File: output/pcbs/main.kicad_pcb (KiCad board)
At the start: 2 copper layers, 142.8 x 177.6 mm, 63 parts

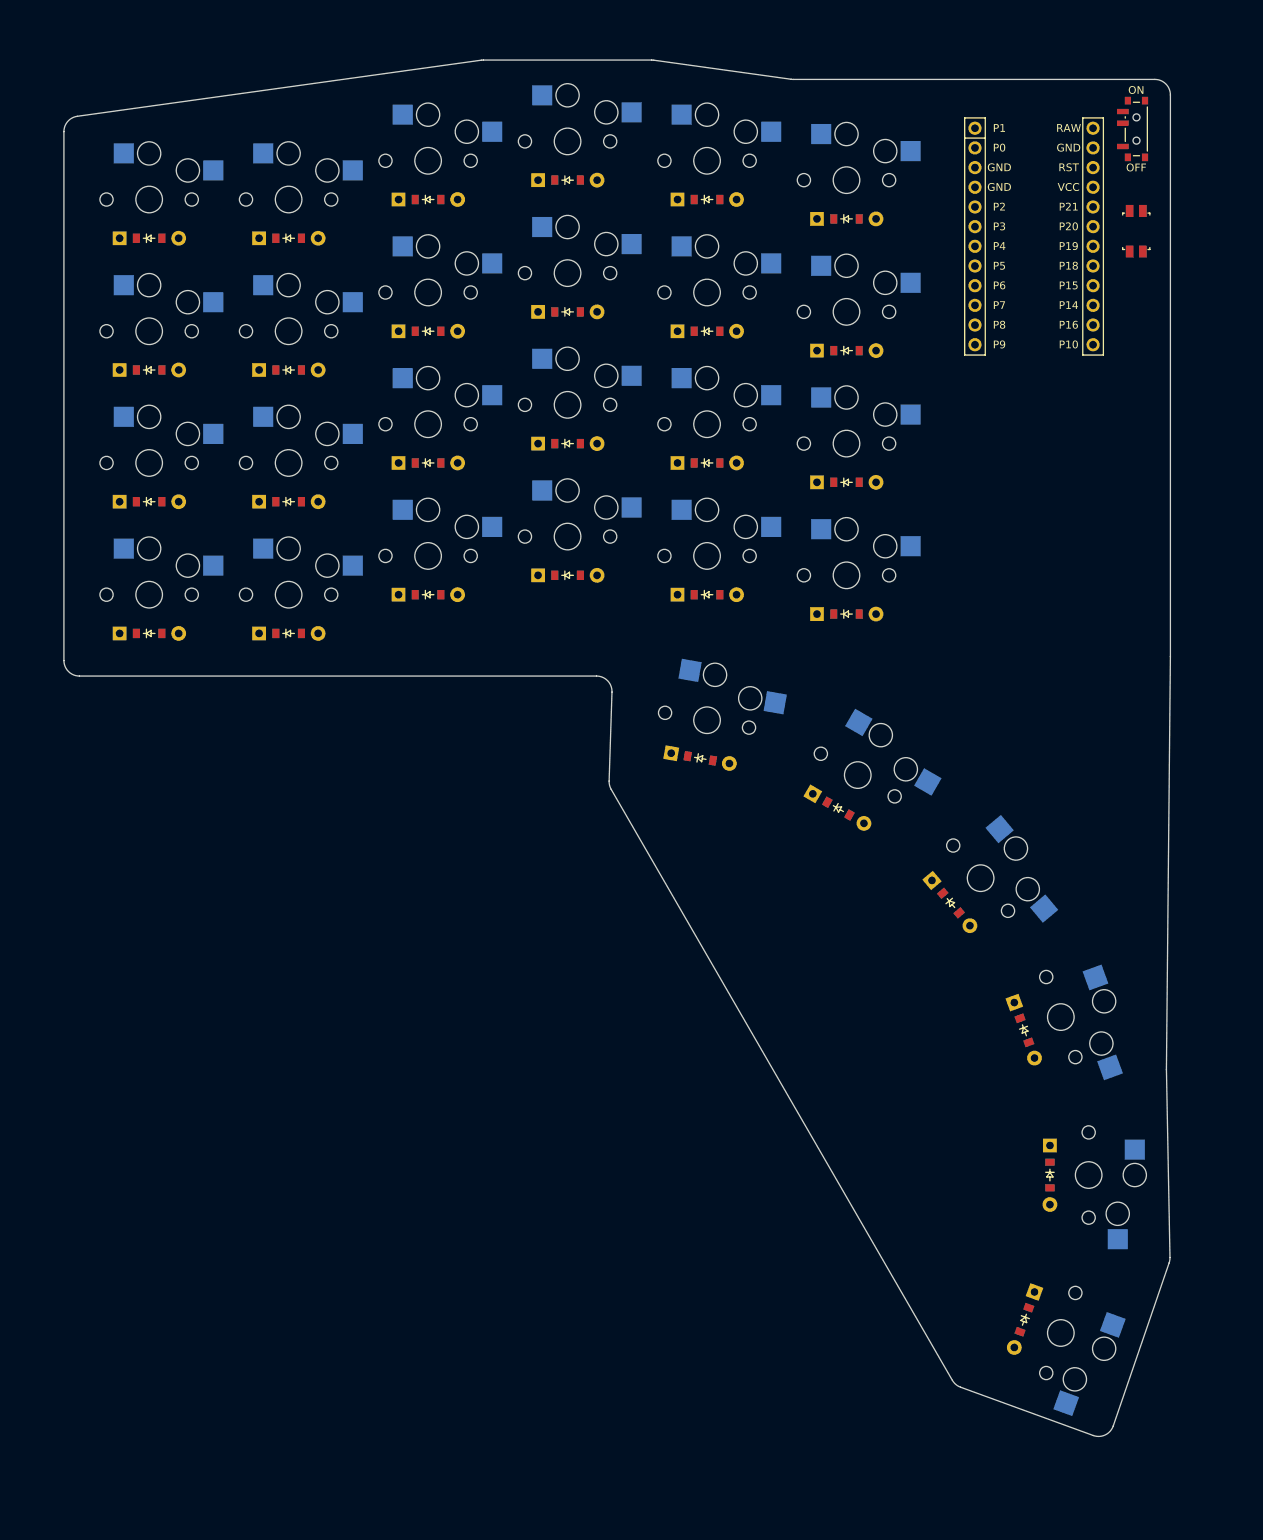
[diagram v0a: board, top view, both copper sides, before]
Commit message: Finished left half maybe
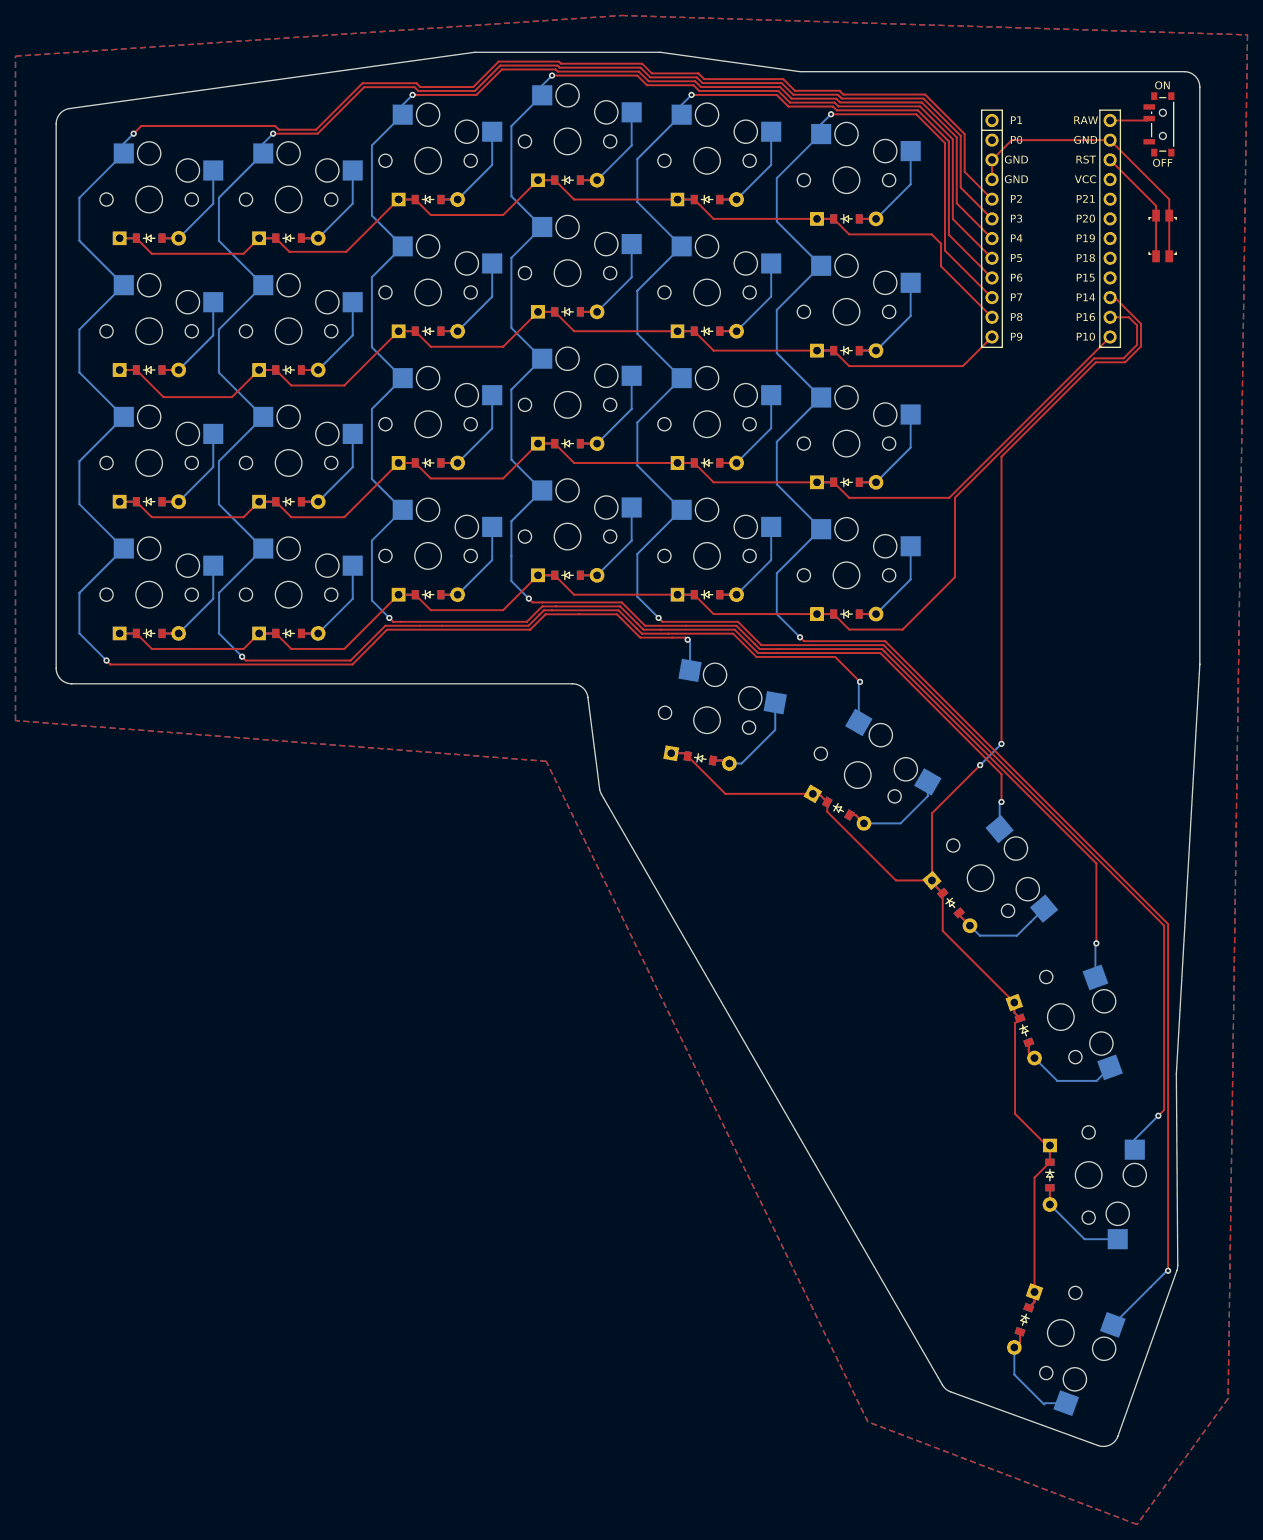
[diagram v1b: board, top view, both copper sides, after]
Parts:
- moved PWR1 3.45 mm to (230.8, 39.3)
- moved RST1 3.45 mm to (230.8, 53.7)
- moved MCU1 2.42 mm to (216.4, 51.5)
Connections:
- D1 pad 1: P5 -> P16
- D10 pad 1: P4 -> P10
- D11 pad 1: P3 -> P9
- D12 pad 1: P2 -> P8
- D13 pad 1: P5 -> P16
- D14 pad 1: P4 -> P10
- D15 pad 1: P3 -> P9
- D16 pad 1: P2 -> P8
- D17 pad 1: P5 -> P16
- D18 pad 1: P4 -> P10
- D19 pad 1: P3 -> P9
- D2 pad 1: P4 -> P10
- D20 pad 1: P2 -> P8
- D21 pad 1: P5 -> P16
- D22 pad 1: P4 -> P10
- D23 pad 1: P3 -> P9
- D24 pad 1: P2 -> P8
- D3 pad 1: P3 -> P9
- D4 pad 1: P2 -> P8
- D5 pad 1: P5 -> P16
- D6 pad 1: P4 -> P10
- D7 pad 1: P3 -> P9
- D8 pad 1: P2 -> P8
- D9 pad 1: P5 -> P16
- S1 pad 1: P6 -> P2
- S10 pad 1: P8 -> P4
- S11 pad 1: P8 -> P4
- S12 pad 1: P8 -> P4
- S13 pad 1: P9 -> P5
- S14 pad 1: P9 -> P5
- S15 pad 1: P9 -> P5
- S16 pad 1: P9 -> P5
- S17 pad 1: P10 -> P6
- S18 pad 1: P10 -> P6
- S19 pad 1: P10 -> P6
- S2 pad 1: P6 -> P2
- S20 pad 1: P10 -> P6
- S21 pad 1: P16 -> P7
- S22 pad 1: P16 -> P7
- S23 pad 1: P16 -> P7
- S24 pad 1: P16 -> P7
- S25 pad 1: P6 -> P2
- S26 pad 1: P7 -> P3
- S27 pad 1: P8 -> P4
- S28 pad 1: P9 -> P5
- S29 pad 1: P10 -> P6
- S3 pad 1: P6 -> P2
- S30 pad 1: P16 -> P7
- S4 pad 1: P6 -> P2
- S5 pad 1: P7 -> P3
- S6 pad 1: P7 -> P3
- S7 pad 1: P7 -> P3
- S8 pad 1: P7 -> P3
- S9 pad 1: P8 -> P4
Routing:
- net P2: track 0.00 -> 295.6 mm, vias 0 -> 3
- net P3: track 0.00 -> 286.6 mm, vias 0 -> 3
- net P4: track 0.00 -> 266.8 mm, vias 0 -> 3
- net P5: track 0.00 -> 255.2 mm, vias 0 -> 3
- net P6: track 0.00 -> 253.6 mm, vias 0 -> 3
- net P7: track 0.00 -> 242.2 mm, vias 0 -> 3
- net P14: track 0.00 -> 208.8 mm, vias 0 -> 2
- net P16: track 0.00 -> 182.9 mm
- net P10: track 0.00 -> 160.4 mm
- net P8: track 0.00 -> 142.5 mm
- net P9: track 0.00 -> 139.3 mm
- net GND: track 0.00 -> 37.0 mm
- net sixth_cluster: track 0.00 -> 16.5 mm
- net fourth_cluster: track 0.00 -> 16.4 mm
- net second_cluster: track 0.00 -> 16.2 mm
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- added copper zone on B.Cu, net GND
- added copper zone on F.Cu, net GND
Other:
- board size 142.8 x 177.6 mm -> 147.6 x 179.9 mm
